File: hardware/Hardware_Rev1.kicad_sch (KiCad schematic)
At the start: 160 parts, among them J1 RJ45_LED_Shielded, J2 6P6C, Q1 BSS138, Q10 AO3401A, Q11 AO3401A, Q12 AO3401A, Q13 BSS138, Q14 BSS138, Q15 BSS138, Q16 AO3401A, Q17 AO3401A, Q18 AO3401A, Q19 BSS138, Q2 BSS138, Q20 BSS138, Q21 BSS138, Q22 AO3401A, Q23 AO3401A, Q24 AO3401A, Q3 BSS138, Q4 AO3401A, Q5 AO3401A, Q6 AO3401A, Q7 BSS138, Q8 BSS138, Q9 BSS138, U1 OKI, U2 Teensy4.1_DEV-16771

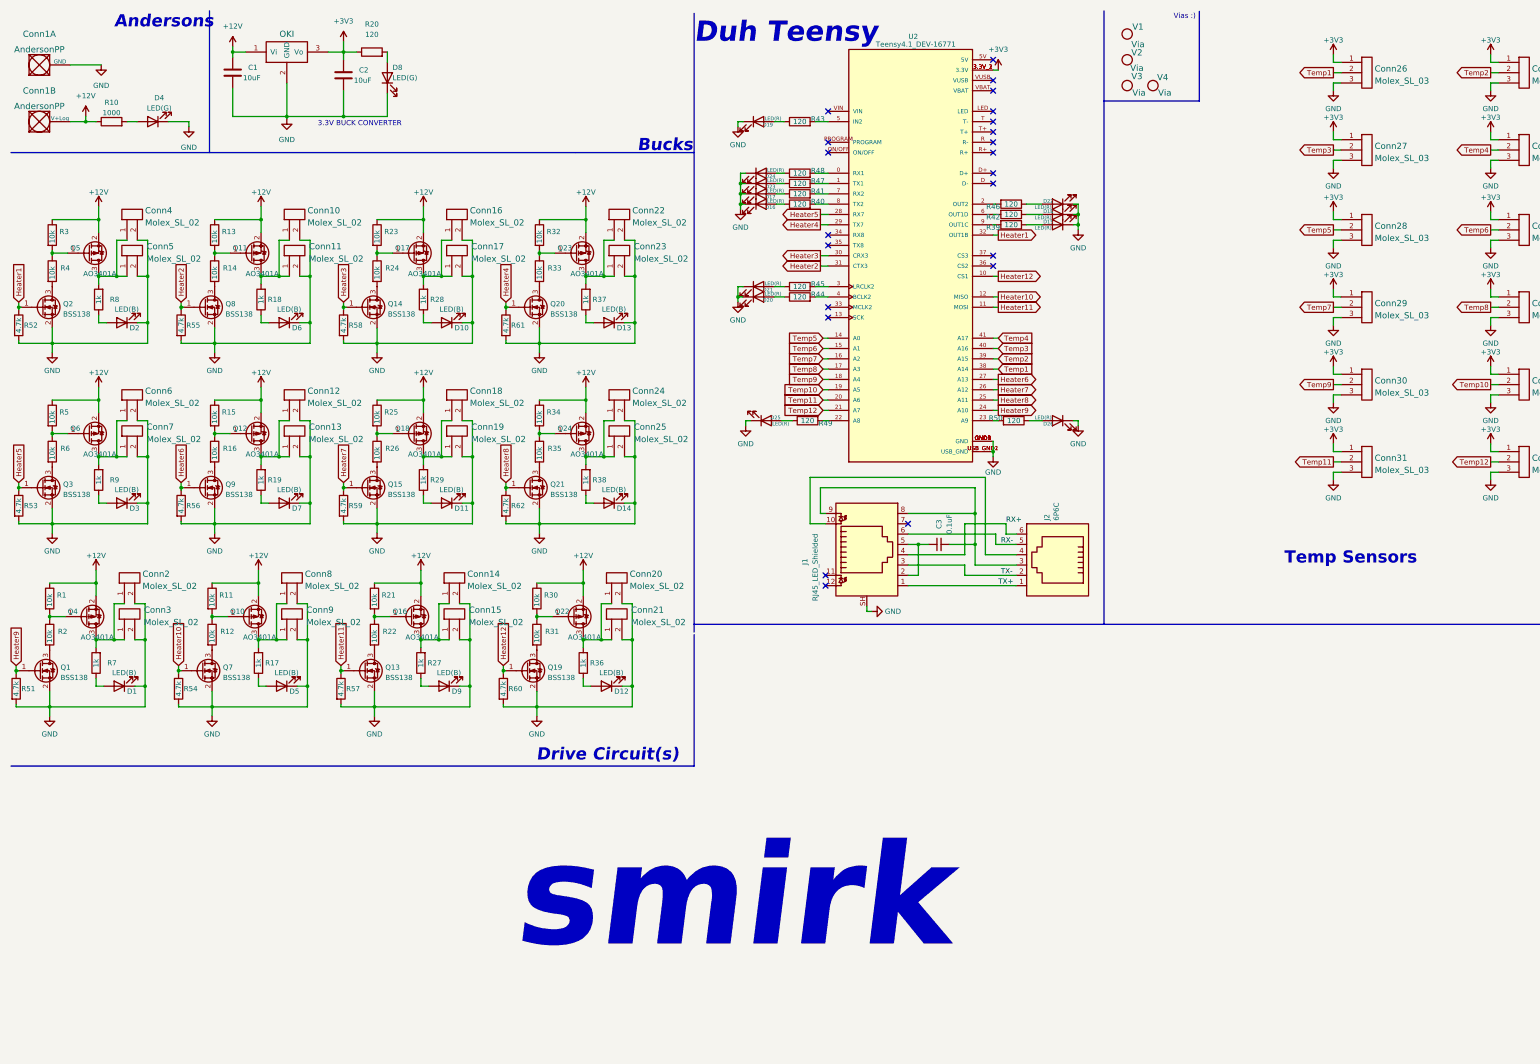
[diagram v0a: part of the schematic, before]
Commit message: Rev2 schematic
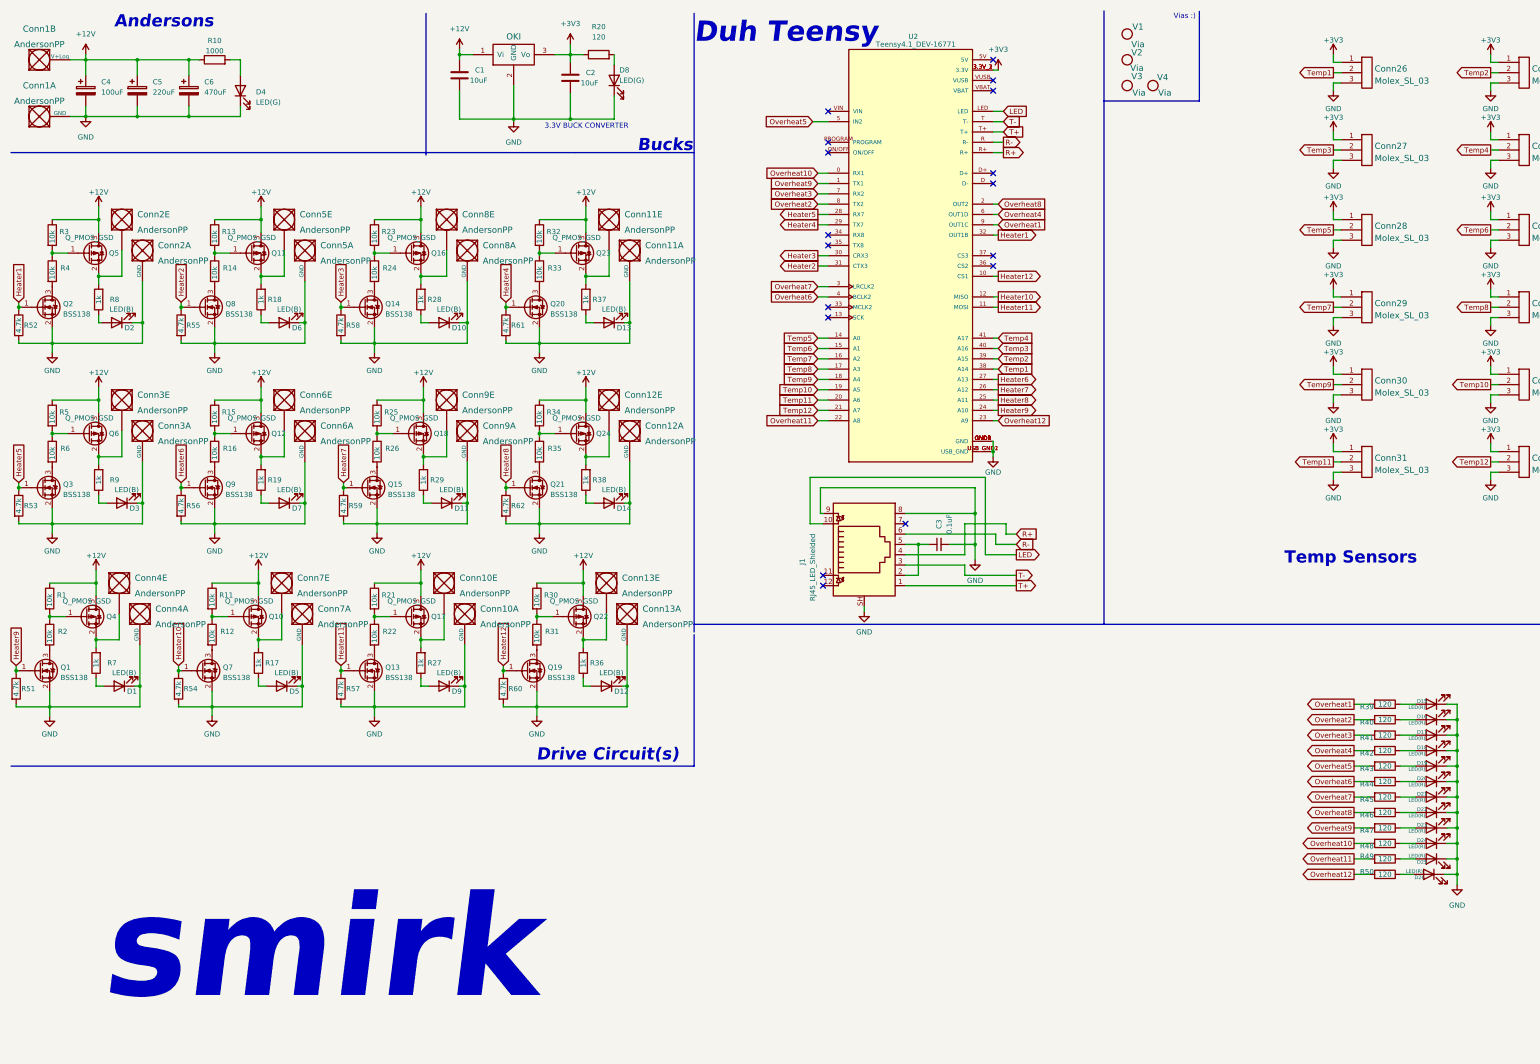
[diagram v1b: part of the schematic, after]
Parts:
- removed Conn10, Conn11, Conn12, Conn13, Conn14, Conn15, Conn16, Conn17, Conn18, Conn19, Conn2, Conn20, Conn21, Conn22, Conn23, Conn24, Conn25, Conn3, Conn4, Conn5, Conn6, Conn7, Conn8, Conn9: Molex_SL_02, MRDT_Connectors:MOLEX_SL_02_Vertical, symbol MRDT_Connectors:Molex_SL_02
- removed J2: 6P6C, Connector_PinHeader_2.00mm:PinHeader_2x03_P2.00mm_Vertical, symbol Connector:6P6C
- removed Q10, Q11, Q12, Q16, Q17, Q18, Q22, Q23, Q24, Q4, Q5, Q6: AO3401A, Package_TO_SOT_SMD:SOT-23, symbol Transistor_FET:AO3401A
- added C4: 100uF, Capacitor_THT:CP_Radial_D6.3mm_P2.50mm, symbol Device:C_Polarized
- added C5: 220uF, Capacitor_THT:CP_Radial_D6.3mm_P2.50mm, symbol Device:C_Polarized
- added C6: 470uF, Capacitor_THT:CP_Radial_D10.0mm_P2.50mm, symbol Device:C_Polarized
- added Conn10, Conn11, Conn12, Conn13, Conn2, Conn3, Conn4, Conn5, Conn6, Conn7, Conn8, Conn9: AndersonPP, MRDT_Connectors:Square_Anderson_2_V_Side_By_Side, symbol MRDT_Connectors:AndersonPP
- added Q10, Q11, Q12, Q16, Q17, Q18, Q22, Q23, Q24, Q4, Q5, Q6: Q_PMOS_GSD, Package_TO_SOT_SMD:SOT-23-3, symbol Device:Q_PMOS_GSD
- U2: footprint MRDT_Shields:Teensy_4_1_Bare -> MRDT_Shields:Teensy_4_1_Ethernet
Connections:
- net RX+ is gone; now on net R+: J1.4
- net RX- is gone; now on net R-: J1.6
- net TX+ is gone; now on net T+: J1.1
- net TX- is gone; now on net T-: J1.3
- net +12V: now also C4.1, C5.1, C6.1, Q10.3 (D), Q11.3 (D), Q12.3 (D), Q16.3 (D), Q17.3 (D), Q18.3 (D), Q22.3 (D), Q23.3 (D), Q24.3 (D), Q4.3 (D), Q5.3 (D), Q6.3 (D)
- net GND: now also C3.2, J1.8, J1.9, C4.2, C5.2, C6.2, Conn10.1 (GND), Conn11.1 (GND), Conn12.1 (GND), Conn13.1 (GND), Conn2.1 (GND), Conn3.1 (GND), Conn4.1 (GND), Conn5.1 (GND), Conn6.1 (GND), Conn7.1 (GND), Conn8.1 (GND), Conn9.1 (GND)
- net at R34.2, R35.1: now also Q24.1 (G)
- net at R30.2, R31.1: now also Q22.1 (G)
- net at R36.2: now also Conn13.1, Q22.2 (S)
- net at R21.2, R22.1: now also Q17.1 (G)
- net Overheat2: now reaches R40.2, U2.8 (TX2)
- net LED: now reaches J1.10
- net LED: now also U2.LED
- net Overheat10: now reaches R48.2, U2.0 (RX1)
- net Overheat9: now reaches R47.2, U2.1 (TX1)
- net Overheat8: now reaches R46.2, U2.2 (OUT2)
- net Overheat11: now reaches R49.2, U2.22 (A8)
- net Overheat12: now reaches R50.2, U2.23 (A9)
- net Overheat7: now reaches R45.2, U2.3 (LRCLK2)
- net Overheat6: now reaches R44.2, U2.4 (BCLK2)
- net Overheat5: now reaches R43.2, U2.5 (IN2)
- net Overheat4: now reaches R42.2, U2.6 (OUT1D)
- net Overheat3: now reaches R41.2, U2.7 (RX2)
- net Overheat1: now reaches R39.2, U2.9 (OUT1C)
- net R-: now reaches U2.R (R-)
- net R+: now reaches U2.R+
- net T-: now reaches U2.T (T-)
- net T+: now reaches U2.T+
- net at R15.2, R16.1: now also Q12.1 (G)
- net at R37.2: now also Conn11.1, Q23.2 (S)
- net at R17.2: now also Conn7.1, Q10.2 (S)
- net at R3.2, R4.1: now also Q5.1 (G)
- net at R8.2: now also Conn2.1, Q5.2 (S)
- net at R27.2: now also Conn10.1, Q17.2 (S)
- net at R5.2, R6.1: now also Q6.1 (G)
- net at R9.2: now also Conn3.1, Q6.2 (S)
- net at R1.2, R2.1: now also Q4.1 (G)
- net at R19.2: now also Conn6.1, Q12.2 (S)
- net at R23.2, R24.1: now also Q16.1 (G)
- net at R28.2: now also Conn8.1, Q16.2 (S)
- net at R32.2, R33.1: now also Q23.1 (G)
- net at R25.2, R26.1: now also Q18.1 (G)
- net at R38.2: now also Conn12.1, Q24.2 (S)
- net at R11.2, R12.1: now also Q10.1 (G)
- net at R18.2: now also Conn5.1, Q11.2 (S)
- net at R7.2: now also Conn4.1, Q4.2 (S)
- net at R13.2, R14.1: now also Q11.1 (G)
- net at R29.2: now also Conn9.1, Q18.2 (S)
- no-connect marks 22 -> 17
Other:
- moved on the sheet: C1, C2, Conn1A, Conn1B, D10, D15, D16, D17, D18, D19, D2, D20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
